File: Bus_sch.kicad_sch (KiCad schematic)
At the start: 9 parts, among them J15 Conn_01x03_Male, J16 Conn_01x20_Male, J17 Conn_01x16_Male, U23 74LS244, U24 74LS373, U25 74LS373, U26 74LS373, U27 74LS245, U28 74LS245

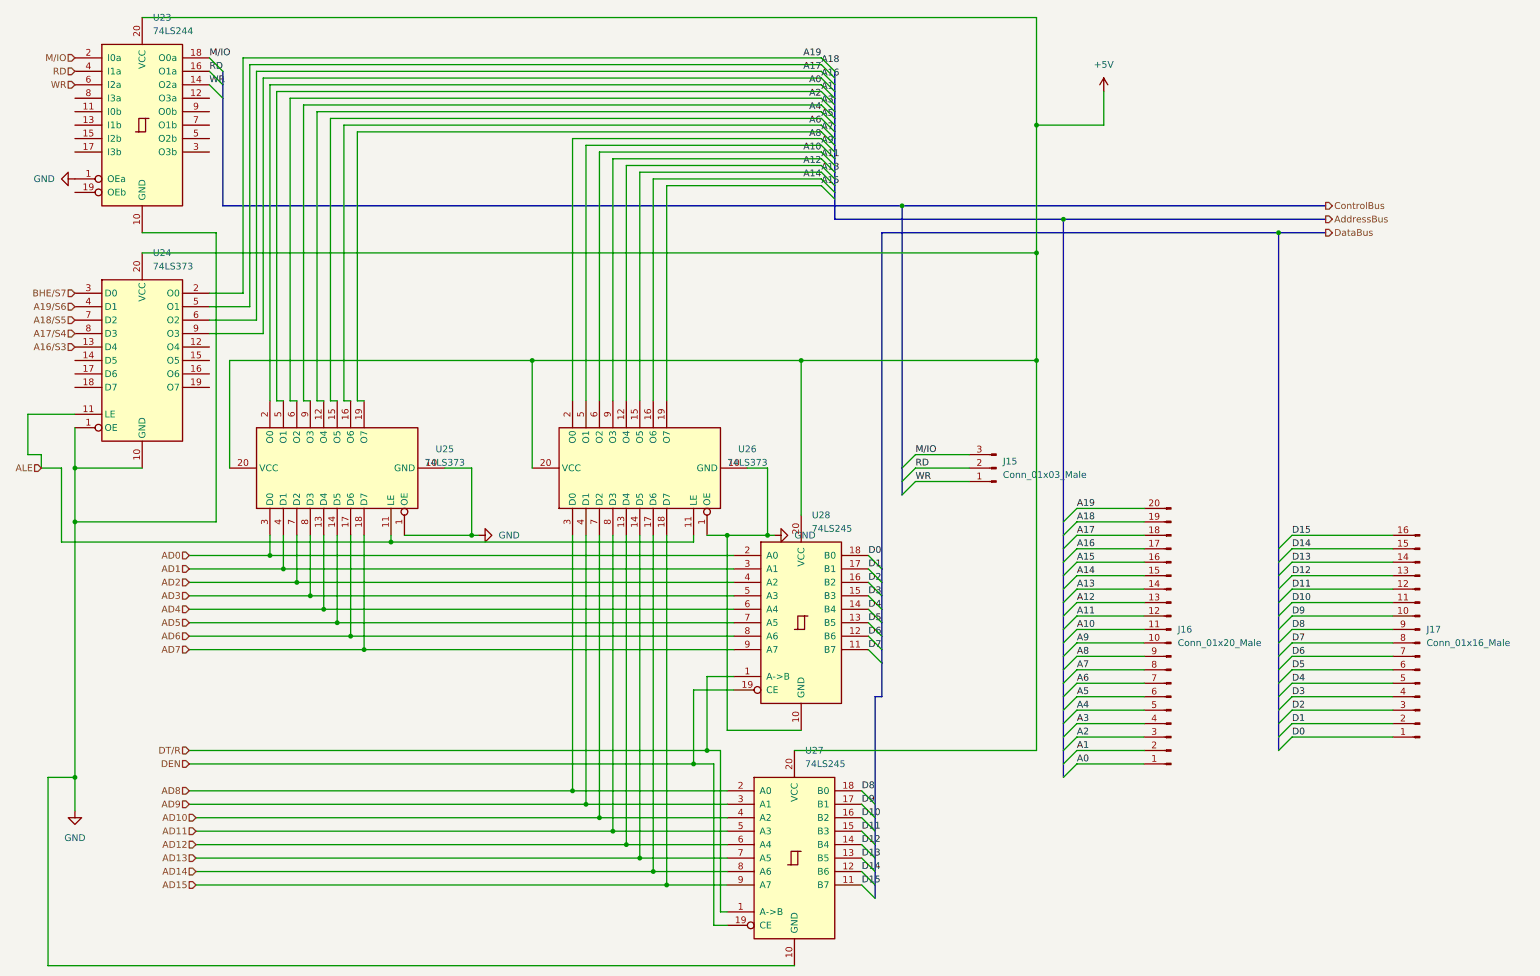
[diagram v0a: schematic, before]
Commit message: Updated PCB
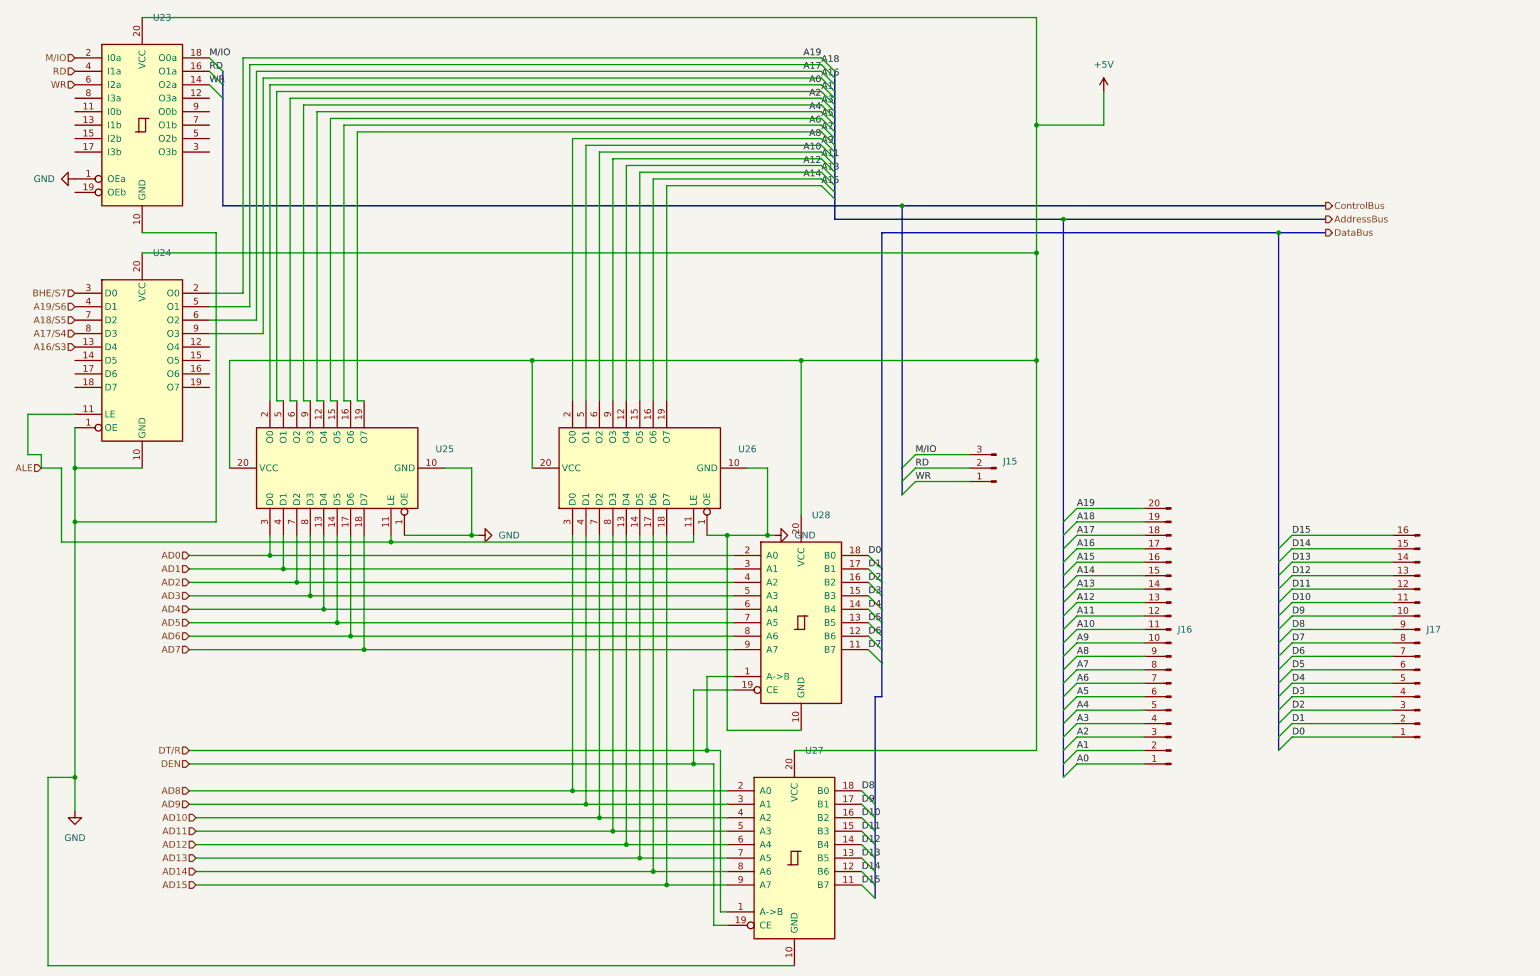
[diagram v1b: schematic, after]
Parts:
- J15: value Conn_01x03_Male -> (none); footprint Connector:FanPinHeader_1x03_P2.54mm_Vertical -> (none)
- J16: value Conn_01x20_Male -> (none); footprint Connector:FanPinHeader_1x03_P2.54mm_Vertical -> (none)
- J17: value Conn_01x16_Male -> (none); footprint Connector:FanPinHeader_1x03_P2.54mm_Vertical -> (none)
- U23: value 74LS244 -> (none); footprint Package_DIP:DIP-20_W7.62mm -> (none)
- U24, U25, U26: value 74LS373 -> (none); footprint Package_DIP:DIP-20_W7.62mm -> (none)
- U27, U28: value 74LS245 -> (none); footprint Package_DIP:DIP-20_W7.62mm -> (none)
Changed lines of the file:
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@@
       (effects (font (size 1.27 1.27)) (justify left))
     )
-    (property "Value" "74LS373" (id 1) (at 38.8494 57.15 0)
-      (effects (font (size 1.27 1.27)) (justify left))
-    )
-    (property "Footprint" "Package_DIP:DIP-20_W7.62mm" (id 2) (at 36.83 74.93 0)
+    (property "Value" "" (id 1) (at 38.8494 57.15 0)
+      (effects (font (size 1.27 1.27)) (justify left))
+    )
+    (property "Footprint" "" (id 2) (at 36.83 74.93 0)
       (effects (font (size 1.27 1.27)) hide)
     )
@@
     (in_bom yes) (on_board yes) (fields_autoplaced)
     (property "Reference" "U26" (id 0) (at 151.13 91.6686 90))
-    (property "Value" "74LS373" (id 1) (at 151.13 94.2086 90))
-    (property "Footprint" "Package_DIP:DIP-20_W7.62mm" (id 2) (at 130.81 95.25 0)
+    (property "Value" "" (id 1) (at 151.13 94.2086 90))
+    (property "Footprint" "" (id 2) (at 130.81 95.25 0)
       (effects (font (size 1.27 1.27)) hide)
     )
@@
       (effects (font (size 1.27 1.27)) (justify left))
     )
-    (property "Value" "74LS245" (id 1) (at 163.3094 106.68 0)
-      (effects (font (size 1.27 1.27)) (justify left))
-    )
-    (property "Footprint" "Package_DIP:DIP-20_W7.62mm" (id 2) (at 161.29 124.46 0)
+    (property "Value" "" (id 1) (at 163.3094 106.68 0)
+      (effects (font (size 1.27 1.27)) (justify left))
+    )
+    (property "Footprint" "" (id 2) (at 161.29 124.46 0)
       (effects (font (size 1.27 1.27)) hide)
     )
@@
       (effects (font (size 1.27 1.27)) (justify right))
     )
-    (property "Value" "Conn_01x16_Male" (id 1) (at 279.4 128.2699 0)
-      (effects (font (size 1.27 1.27)) (justify right))
-    )
-    (property "Footprint" "Connector:FanPinHeader_1x03_P2.54mm_Vertical" (id 2) (at 278.13 128.27 0)
+    (property "Value" "" (id 1) (at 279.4 128.2699 0)
+      (effects (font (size 1.27 1.27)) (justify right))
+    )
+    (property "Footprint" "" (id 2) (at 278.13 128.27 0)
       (effects (font (size 1.27 1.27)) hide)
     )
@@
   (symbol (lib_id "power:+5V") (at 218.44 24.13 0) (unit 1)
     (in_bom yes) (on_board yes) (fields_autoplaced)
-    (property "Reference" "#PWR?" (id 0) (at 218.44 27.94 0)
+    (property "Reference" "#PWR0131" (id 0) (at 218.44 27.94 0)
       (effects (font (size 1.27 1.27)) hide)
     )
@@
       (effects (font (size 1.27 1.27)) (justify right))
     )
-    (property "Value" "Conn_01x20_Male" (id 1) (at 232.41 128.2699 0)
-      (effects (font (size 1.27 1.27)) (justify right))
-    )
-    (property "Footprint" "Connector:FanPinHeader_1x03_P2.54mm_Vertical" (id 2) (at 231.14 128.27 0)
+    (property "Value" "" (id 1) (at 232.41 128.2699 0)
+      (effects (font (size 1.27 1.27)) (justify right))
+    )
+    (property "Footprint" "" (id 2) (at 231.14 128.27 0)
       (effects (font (size 1.27 1.27)) hide)
     )
@@
     (in_bom yes) (on_board yes) (fields_autoplaced)
     (property "Reference" "U25" (id 0) (at 93.98 91.6686 90))
-    (property "Value" "74LS373" (id 1) (at 93.98 94.2086 90))
-    (property "Footprint" "Package_DIP:DIP-20_W7.62mm" (id 2) (at 73.66 95.25 0)
+    (property "Value" "" (id 1) (at 93.98 94.2086 90))
+    (property "Footprint" "" (id 2) (at 73.66 95.25 0)
       (effects (font (size 1.27 1.27)) hide)
     )
@@
       (effects (font (size 1.27 1.27)) (justify left))
     )
-    (property "Value" "74LS245" (id 1) (at 162.0394 151.13 0)
-      (effects (font (size 1.27 1.27)) (justify left))
-    )
-    (property "Footprint" "Package_DIP:DIP-20_W7.62mm" (id 2) (at 160.02 168.91 0)
+    (property "Value" "" (id 1) (at 162.0394 151.13 0)
+      (effects (font (size 1.27 1.27)) (justify left))
+    )
+    (property "Footprint" "" (id 2) (at 160.02 168.91 0)
       (effects (font (size 1.27 1.27)) hide)
     )
@@
       (effects (font (size 1.27 1.27)) (justify right))
     )
-    (property "Value" "Conn_01x03_Male" (id 1) (at 199.39 96.5199 0)
-      (effects (font (size 1.27 1.27)) (justify right))
-    )
-    (property "Footprint" "Connector:FanPinHeader_1x03_P2.54mm_Vertical" (id 2) (at 198.12 95.25 0)
+    (property "Value" "" (id 1) (at 199.39 96.5199 0)
+      (effects (font (size 1.27 1.27)) (justify right))
+    )
+    (property "Footprint" "" (id 2) (at 198.12 95.25 0)
       (effects (font (size 1.27 1.27)) hide)
     )
@@
       (effects (font (size 1.27 1.27)) (justify left))
     )
-    (property "Value" "74LS244" (id 1) (at 38.8494 12.7 0)
-      (effects (font (size 1.27 1.27)) (justify left))
-    )
-    (property "Footprint" "Package_DIP:DIP-20_W7.62mm" (id 2) (at 36.83 30.48 0)
-      (effects (font (size 1.27 1.27)) hide)
-    )
+    (property "Value" "" (id 1) (at 38.8494 12.7 0)
+      (effects (font (size 1.27 1.27)) (justify left))
+    )
+    (property "Footprint" "" (id 2) (at 36.83 30.48 0)
+      (effects (font (size 1.27 1.27)) hide)
+    )

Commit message: PCB wiring
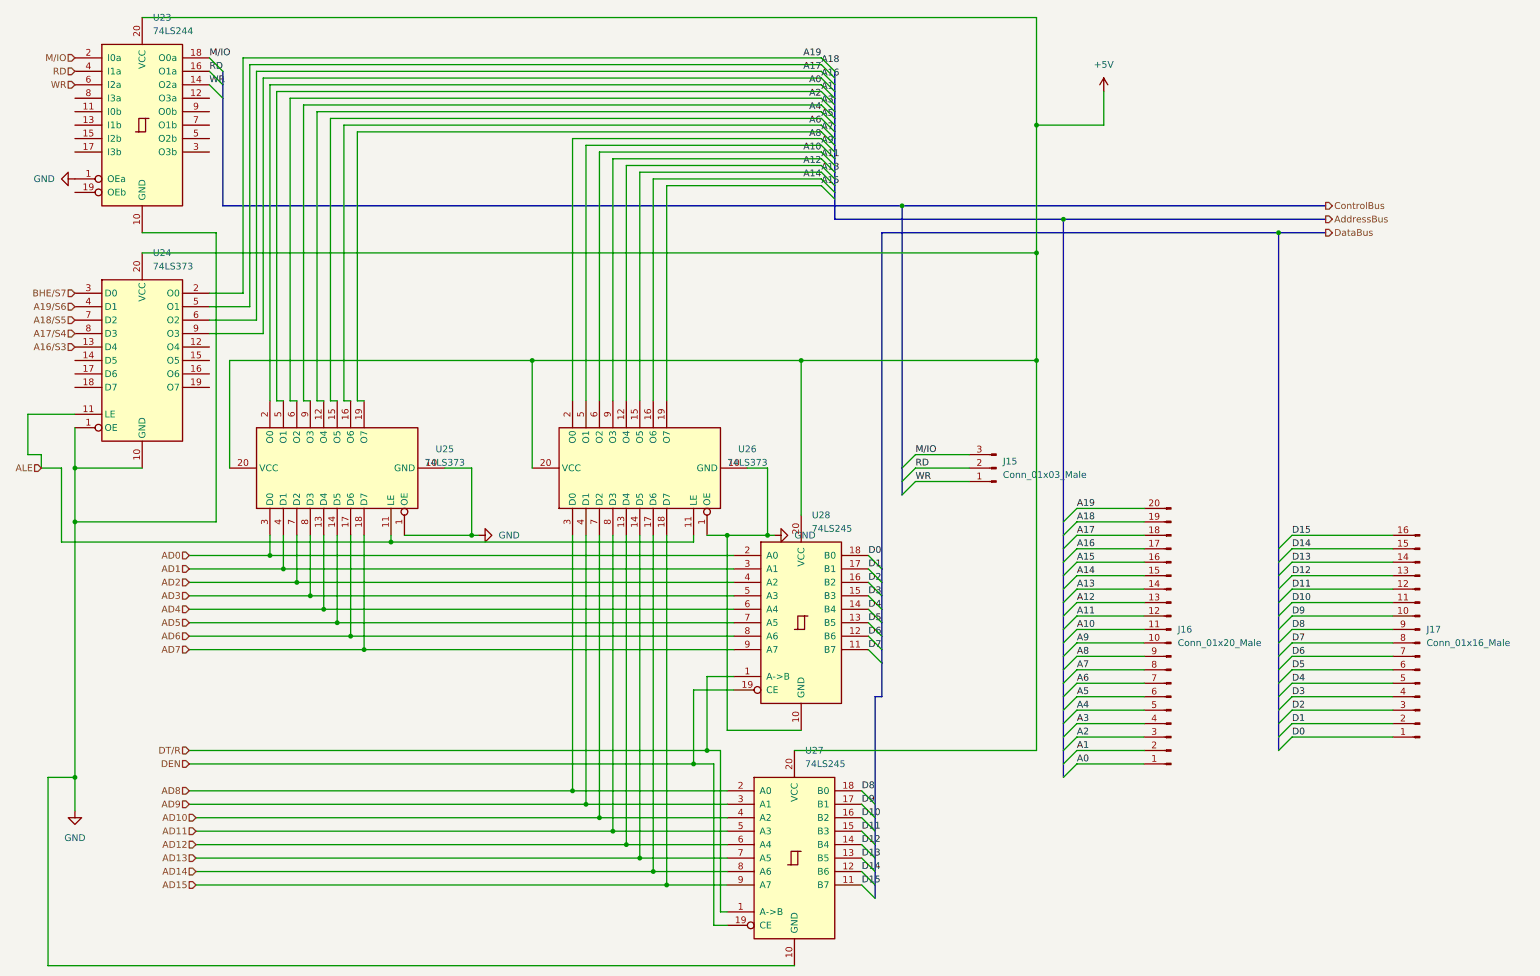
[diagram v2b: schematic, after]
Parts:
- J15: value (none) -> Conn_01x03_Male; footprint (none) -> Connector:FanPinHeader_1x03_P2.54mm_Vertical
- J16: value (none) -> Conn_01x20_Male; footprint (none) -> Connector:FanPinHeader_1x03_P2.54mm_Vertical
- J17: value (none) -> Conn_01x16_Male; footprint (none) -> Connector:FanPinHeader_1x03_P2.54mm_Vertical
- U23: value (none) -> 74LS244; footprint (none) -> Package_DIP:DIP-20_W7.62mm
- U24, U25, U26: value (none) -> 74LS373; footprint (none) -> Package_DIP:DIP-20_W7.62mm
- U27, U28: value (none) -> 74LS245; footprint (none) -> Package_DIP:DIP-20_W7.62mm
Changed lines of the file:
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@@
       (effects (font (size 1.27 1.27)) (justify left))
     )
-    (property "Value" "" (id 1) (at 38.8494 57.15 0)
-      (effects (font (size 1.27 1.27)) (justify left))
-    )
-    (property "Footprint" "" (id 2) (at 36.83 74.93 0)
+    (property "Value" "74LS373" (id 1) (at 38.8494 57.15 0)
+      (effects (font (size 1.27 1.27)) (justify left))
+    )
+    (property "Footprint" "Package_DIP:DIP-20_W7.62mm" (id 2) (at 36.83 74.93 0)
       (effects (font (size 1.27 1.27)) hide)
     )
@@
     (in_bom yes) (on_board yes) (fields_autoplaced)
     (property "Reference" "U26" (id 0) (at 151.13 91.6686 90))
-    (property "Value" "" (id 1) (at 151.13 94.2086 90))
-    (property "Footprint" "" (id 2) (at 130.81 95.25 0)
+    (property "Value" "74LS373" (id 1) (at 151.13 94.2086 90))
+    (property "Footprint" "Package_DIP:DIP-20_W7.62mm" (id 2) (at 130.81 95.25 0)
       (effects (font (size 1.27 1.27)) hide)
     )
@@
       (effects (font (size 1.27 1.27)) (justify left))
     )
-    (property "Value" "" (id 1) (at 163.3094 106.68 0)
-      (effects (font (size 1.27 1.27)) (justify left))
-    )
-    (property "Footprint" "" (id 2) (at 161.29 124.46 0)
+    (property "Value" "74LS245" (id 1) (at 163.3094 106.68 0)
+      (effects (font (size 1.27 1.27)) (justify left))
+    )
+    (property "Footprint" "Package_DIP:DIP-20_W7.62mm" (id 2) (at 161.29 124.46 0)
       (effects (font (size 1.27 1.27)) hide)
     )
@@
       (effects (font (size 1.27 1.27)) (justify right))
     )
-    (property "Value" "" (id 1) (at 279.4 128.2699 0)
-      (effects (font (size 1.27 1.27)) (justify right))
-    )
-    (property "Footprint" "" (id 2) (at 278.13 128.27 0)
+    (property "Value" "Conn_01x16_Male" (id 1) (at 279.4 128.2699 0)
+      (effects (font (size 1.27 1.27)) (justify right))
+    )
+    (property "Footprint" "Connector:FanPinHeader_1x03_P2.54mm_Vertical" (id 2) (at 278.13 128.27 0)
       (effects (font (size 1.27 1.27)) hide)
     )
@@
       (effects (font (size 1.27 1.27)) (justify right))
     )
-    (property "Value" "" (id 1) (at 232.41 128.2699 0)
-      (effects (font (size 1.27 1.27)) (justify right))
-    )
-    (property "Footprint" "" (id 2) (at 231.14 128.27 0)
+    (property "Value" "Conn_01x20_Male" (id 1) (at 232.41 128.2699 0)
+      (effects (font (size 1.27 1.27)) (justify right))
+    )
+    (property "Footprint" "Connector:FanPinHeader_1x03_P2.54mm_Vertical" (id 2) (at 231.14 128.27 0)
       (effects (font (size 1.27 1.27)) hide)
     )
@@
     (in_bom yes) (on_board yes) (fields_autoplaced)
     (property "Reference" "U25" (id 0) (at 93.98 91.6686 90))
-    (property "Value" "" (id 1) (at 93.98 94.2086 90))
-    (property "Footprint" "" (id 2) (at 73.66 95.25 0)
+    (property "Value" "74LS373" (id 1) (at 93.98 94.2086 90))
+    (property "Footprint" "Package_DIP:DIP-20_W7.62mm" (id 2) (at 73.66 95.25 0)
       (effects (font (size 1.27 1.27)) hide)
     )
@@
       (effects (font (size 1.27 1.27)) (justify left))
     )
-    (property "Value" "" (id 1) (at 162.0394 151.13 0)
-      (effects (font (size 1.27 1.27)) (justify left))
-    )
-    (property "Footprint" "" (id 2) (at 160.02 168.91 0)
+    (property "Value" "74LS245" (id 1) (at 162.0394 151.13 0)
+      (effects (font (size 1.27 1.27)) (justify left))
+    )
+    (property "Footprint" "Package_DIP:DIP-20_W7.62mm" (id 2) (at 160.02 168.91 0)
       (effects (font (size 1.27 1.27)) hide)
     )
@@
       (effects (font (size 1.27 1.27)) (justify right))
     )
-    (property "Value" "" (id 1) (at 199.39 96.5199 0)
-      (effects (font (size 1.27 1.27)) (justify right))
-    )
-    (property "Footprint" "" (id 2) (at 198.12 95.25 0)
+    (property "Value" "Conn_01x03_Male" (id 1) (at 199.39 96.5199 0)
+      (effects (font (size 1.27 1.27)) (justify right))
+    )
+    (property "Footprint" "Connector:FanPinHeader_1x03_P2.54mm_Vertical" (id 2) (at 198.12 95.25 0)
       (effects (font (size 1.27 1.27)) hide)
     )
@@
       (effects (font (size 1.27 1.27)) (justify left))
     )
-    (property "Value" "" (id 1) (at 38.8494 12.7 0)
-      (effects (font (size 1.27 1.27)) (justify left))
-    )
-    (property "Footprint" "" (id 2) (at 36.83 30.48 0)
-      (effects (font (size 1.27 1.27)) hide)
-    )
+    (property "Value" "74LS244" (id 1) (at 38.8494 12.7 0)
+      (effects (font (size 1.27 1.27)) (justify left))
+    )
+    (property "Footprint" "Package_DIP:DIP-20_W7.62mm" (id 2) (at 36.83 30.48 0)
+      (effects (font (size 1.27 1.27)) hide)
+    )

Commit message: pcb wiring
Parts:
- J16, J17: footprint Connector:FanPinHeader_1x03_P2.54mm_Vertical -> (none)
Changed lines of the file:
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@@
       (effects (font (size 1.27 1.27)) (justify right))
     )
-    (property "Footprint" "Connector:FanPinHeader_1x03_P2.54mm_Vertical" (id 2) (at 278.13 128.27 0)
+    (property "Footprint" "" (id 2) (at 278.13 128.27 0)
       (effects (font (size 1.27 1.27)) hide)
     )
@@
       (effects (font (size 1.27 1.27)) (justify right))
     )
-    (property "Footprint" "Connector:FanPinHeader_1x03_P2.54mm_Vertical" (id 2) (at 231.14 128.27 0)
+    (property "Footprint" "" (id 2) (at 231.14 128.27 0)
       (effects (font (size 1.27 1.27)) hide)
     )
